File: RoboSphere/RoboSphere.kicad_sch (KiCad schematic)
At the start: 20 parts, among them SW1 SW_Push, U1 RASPBERRY_PI_ZERO_2_W, U2 DRV8833PWP, U3 ADS1115IDGS, U5 L7806

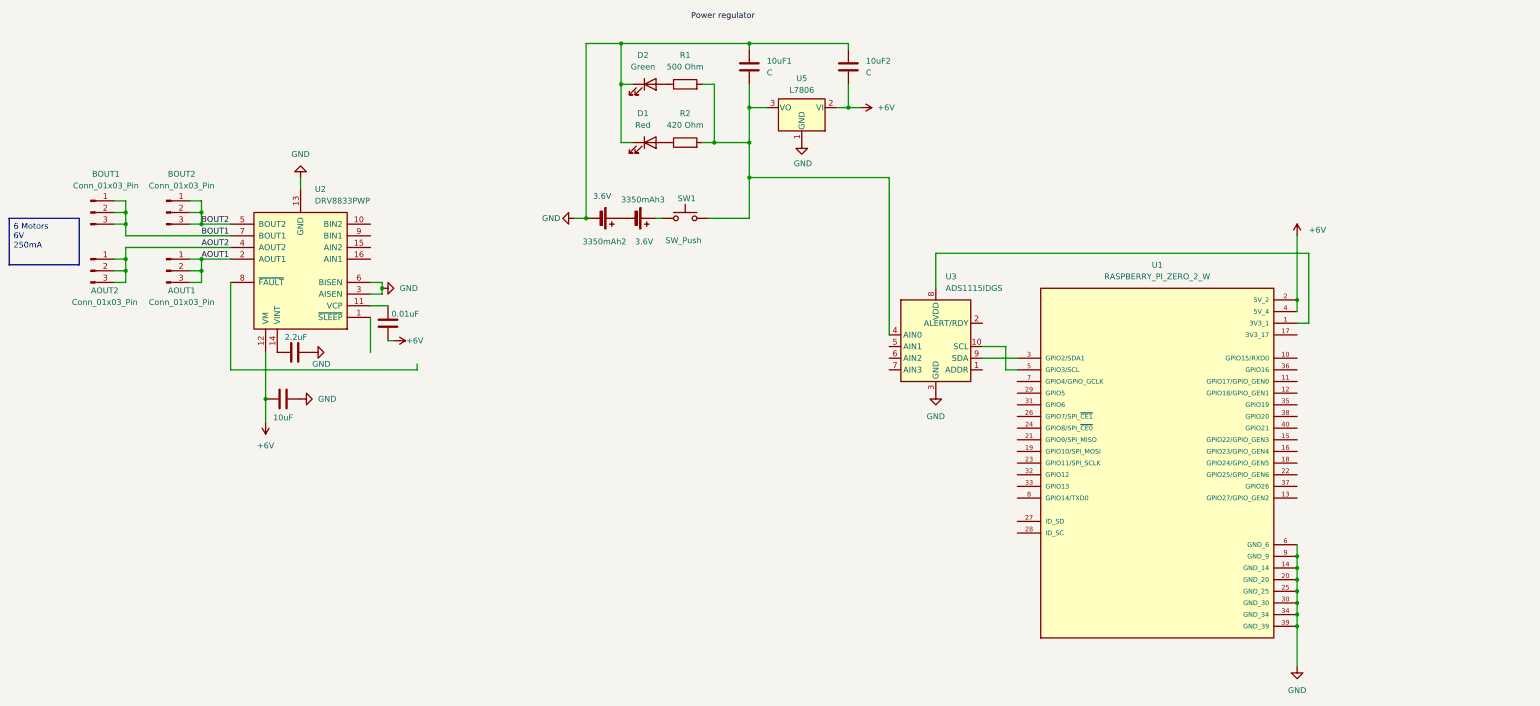
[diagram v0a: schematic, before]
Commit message: Update
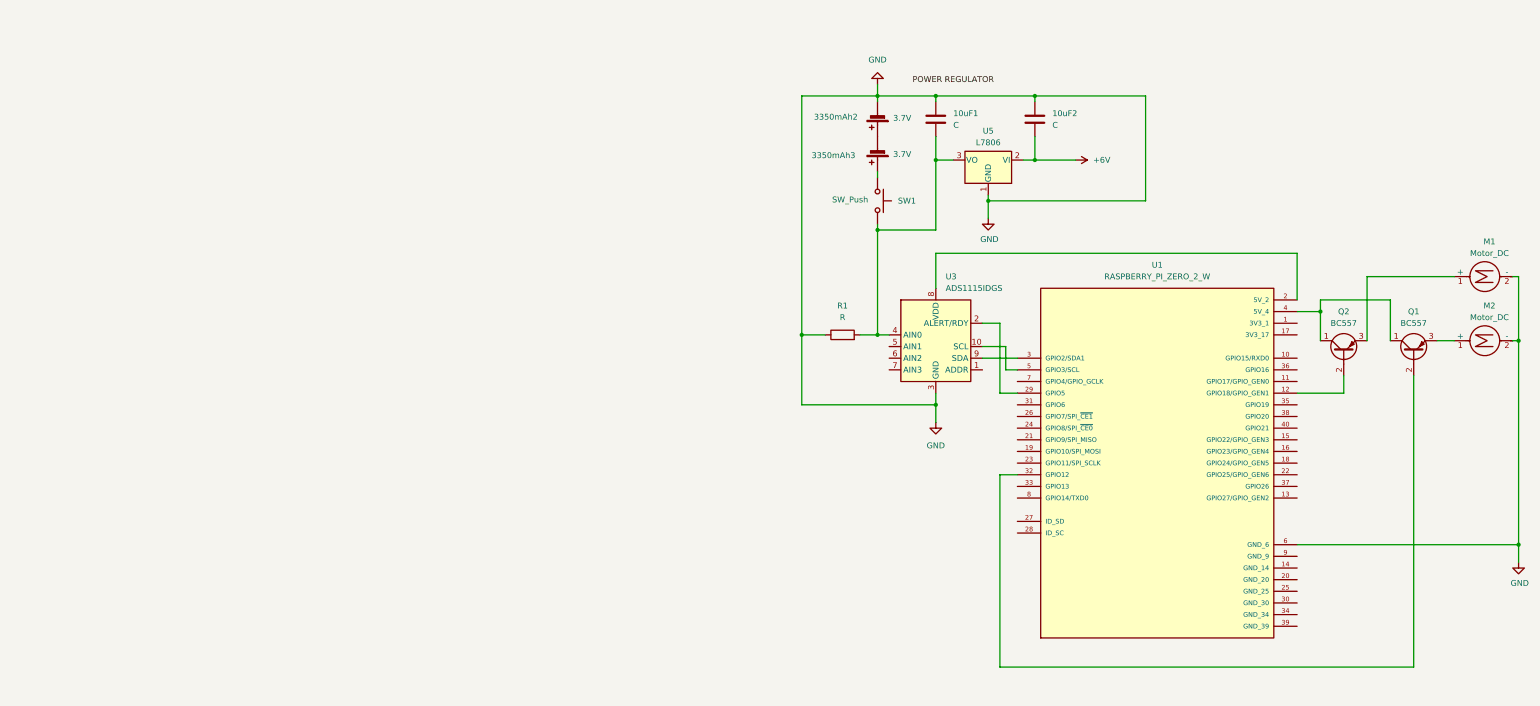
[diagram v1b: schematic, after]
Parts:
- removed AOUT1, AOUT2, BOUT1, BOUT2: Conn_01x03_Pin, Connector_PinHeader_2.54mm:PinHeader_1x03_P2.54mm_Vertical_SMD_Pin1Left, symbol Connector:Conn_01x03_Pin
- removed C1: 0.01uF, Capacitor_SMD:C_0805_2012Metric, symbol Device:C
- removed C2: 10uF, Capacitor_SMD:C_0805_2012Metric, symbol Device:C
- removed C3: 2.2uF, Capacitor_SMD:C_0805_2012Metric, symbol Device:C
- removed D1: Red, symbol Device:LED
- removed D2: Green, symbol Device:LED
- removed R2: 420 Ohm, symbol Device:R
- removed U2: DRV8833PWP, Package_SO:HTSSOP-16-1EP_4.4x5mm_P0.65mm_EP3.4x5mm_Mask2.46x2.31mm_ThermalVias, symbol Driver_Motor:DRV8833PWP
- added M1, M2: Motor_DC, symbol Motor:Motor_DC
- added Q1, Q2: BC557, Package_TO_SOT_THT:TO-92_Inline, symbol Transistor_BJT:BC557
- 3350mAh2, 3350mAh3: value 3.6V -> 3.7V
- R1: value 500 Ohm -> R
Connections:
- net +6V: no longer U1.2 (5V_2), U1.4 (5V_4)
- net GND: now also R1.1, M1.2 (-), M2.2 (-); no longer U1.14 (GND_14), U1.20 (GND_20), U1.25 (GND_25), U1.30 (GND_30), U1.34 (GND_34), U1.39 (GND_39), U1.9 (GND_9)
- net at U1.1 (3V3_1): no longer U3.8 (VDD)
- net at U1.12 (GPIO18/GPIO_GEN1): now also Q2.2 (B)
- net at U1.29 (GPIO5): now also U3.2 (ALERT/RDY)
- net at U1.32 (GPIO12): now also Q1.2 (B)
- new net: U1.2 (5V_2), U3.8 (VDD)
- new net: Q1.1 (C), Q2.1 (C), U1.4 (5V_4)
- new net: M2.1 (+), Q1.3 (E)
- new net: M1.1 (+), Q2.3 (E)
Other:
- moved on the sheet: 10uF1, 10uF2, 3350mAh2, 3350mAh3, SW1, U5
